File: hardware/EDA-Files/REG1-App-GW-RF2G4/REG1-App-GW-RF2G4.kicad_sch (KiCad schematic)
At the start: 4 parts, among them J1 REG1_App_Connector, U1 E01-ML01DP5, U2 E01-2G4M27S, U3 E07-M1101D-TH

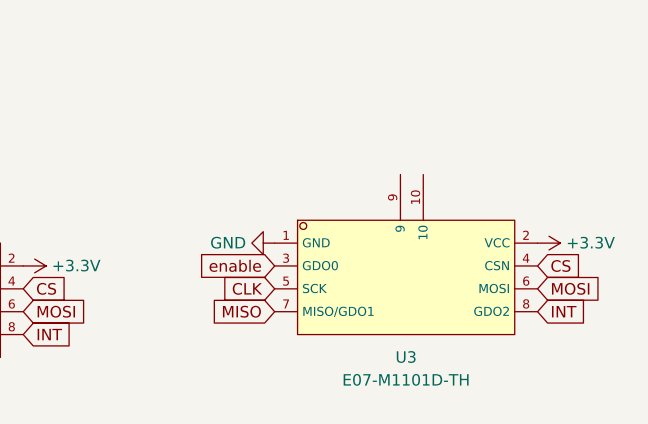
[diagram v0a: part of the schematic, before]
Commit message: wip GW RF
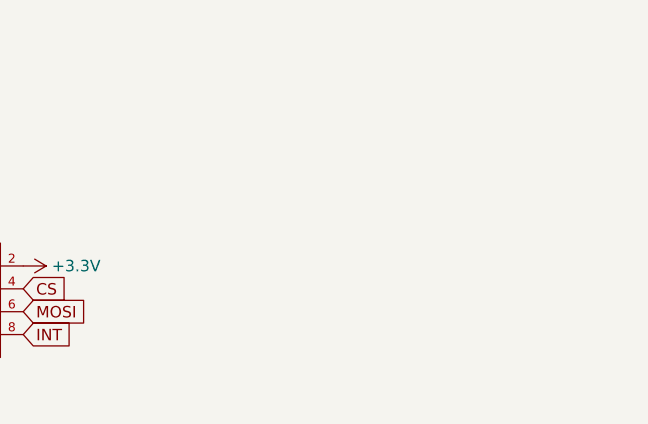
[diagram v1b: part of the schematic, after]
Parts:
- removed U3: E07-M1101D-TH, EasyEDALib:WIRELM-TH_E07-M1101D-TH, symbol EasyEDALib:E07-M1101D-TH
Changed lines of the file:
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@@
     (company "OpenKNX")
     (comment 1 "by Ing-Dom <dom@ing-dom.de>")
+    (comment 2 "OpenKNX Open Hardware under CC BY-NC-SA 4.0")
     (comment 3 "REG1-Application PCB for a 2.4GHz RF module featuring NRF24L01+ chipset")
     (comment 4 "https://OpenKNX.de")
@@
     )
   )
-  (global_label "MOSI" (shape input) (at 237.49 85.09 0) (fields_autoplaced)
-    (effects (font (size 1.27 1.27)) (justify left))
-    (property "Intersheetrefs" "${INTERSHEET_REFS}" (at 244.4172 85.09 0)
-      (effects (font (size 1.27 1.27)) (justify left) hide)
-    )
-  )
-  (global_label "INT" (shape input) (at 237.49 87.63 0) (fields_autoplaced)
-    (effects (font (size 1.27 1.27)) (justify left))
-    (property "Intersheetrefs" "${INTERSHEET_REFS}" (at 242.7239 87.63 0)
-      (effects (font (size 1.27 1.27)) (justify left) hide)
-    )
-  )
   (global_label "INT" (shape input) (at 87.63 45.72 0) (fields_autoplaced)
     (effects (font (size 1.27 1.27)) (justify left))
@@
     )
   )
-  (global_label "enable" (shape input) (at 208.28 82.55 180) (fields_autoplaced)
-    (effects (font (size 1.27 1.27)) (justify right))
-    (property "Intersheetrefs" "${INTERSHEET_REFS}" (at 199.6596 82.55 0)
-      (effects (font (size 1.27 1.27)) (justify right) hide)
-    )
-  )
   (global_label "enable" (shape input) (at 156.21 38.1 180) (fields_autoplaced)
     (effects (font (size 1.27 1.27)) (justify right))
@@
     )
   )
-  (global_label "CS" (shape input) (at 237.49 82.55 0) (fields_autoplaced)
-    (effects (font (size 1.27 1.27)) (justify left))
-    (property "Intersheetrefs" "${INTERSHEET_REFS}" (at 242.3005 82.55 0)
-      (effects (font (size 1.27 1.27)) (justify left) hide)
-    )
-  )
   (global_label "CS" (shape input) (at 87.63 55.88 0) (fields_autoplaced)
     (effects (font (size 1.27 1.27)) (justify left))
@@
     )
   )
-  (global_label "CLK" (shape input) (at 208.28 85.09 180) (fields_autoplaced)
-    (effects (font (size 1.27 1.27)) (justify right))
-    (property "Intersheetrefs" "${INTERSHEET_REFS}" (at 202.3809 85.09 0)
-      (effects (font (size 1.27 1.27)) (justify right) hide)
-    )
-  )
   (global_label "MISO" (shape input) (at 146.05 90.17 180) (fields_autoplaced)
     (effects (font (size 1.27 1.27)) (justify right))
     (property "Intersheetrefs" "${INTERSHEET_REFS}" (at 139.1228 90.17 0)
-      (effects (font (size 1.27 1.27)) (justify right) hide)
-    )
-  )
-  (global_label "MISO" (shape input) (at 208.28 87.63 180) (fields_autoplaced)
-    (effects (font (size 1.27 1.27)) (justify right))
-    (property "Intersheetrefs" "${INTERSHEET_REFS}" (at 201.3528 87.63 0)
       (effects (font (size 1.27 1.27)) (justify right) hide)
     )
@@
     )
   )
-  (symbol (lib_id "power:+3.3V") (at 237.49 80.01 270) (unit 1)
-    (in_bom yes) (on_board yes) (dnp no) (fields_autoplaced)
-    (property "Reference" "#PWR08" (at 233.68 80.01 0)
-      (effects (font (size 1.27 1.27)) hide)
-    )
-    (property "Value" "+3.3V" (at 240.665 80.01 90)
-      (effects (font (size 1.27 1.27)) (justify left))
-    )
-    (property "Footprint" "" (at 237.49 80.01 0)
-      (effects (font (size 1.27 1.27)) hide)
-    )
-    (property "Datasheet" "" (at 237.49 80.01 0)
-      (effects (font (size 1.27 1.27)) hide)
-    )
-    (pin "1")
-    (instances
-      (project "REG1-App-GW-RF2G4"
-        (path "/8b58e694-2557-4422-b559-288aecb40f90"
-          (reference "#PWR08") (unit 1)
-        )
-      )
-    )
-  )
   (symbol (lib_id "power:GND") (at 87.63 58.42 90) (unit 1)
     (in_bom yes) (on_board yes) (dnp no) (fields_autoplaced)
@@
     )
   )
-  (symbol (lib_id "EasyEDALib:E07-M1101D-TH") (at 223.52 83.82 0) (unit 1)
-    (in_bom yes) (on_board yes) (dnp no) (fields_autoplaced)
-    (property "Reference" "U3" (at 222.885 92.71 0)
-      (effects (font (size 1.27 1.27)))
-    )
-    (property "Value" "E07-M1101D-TH" (at 222.885 95.25 0)
-      (effects (font (size 1.27 1.27)))
-    )
-    (property "Footprint" "EasyEDALib:WIRELM-TH_E07-M1101D-TH" (at 223.52 93.98 0)
-      (effects (font (size 1.27 1.27) italic) hide)
-    )
-    (property "Datasheet" "https://item.szlcsc.com/109768.html" (at 221.234 83.693 0)
-      (effects (font (size 1.27 1.27)) (justify left) hide)
-    )
-    (property "LCSC" "C108549" (at 223.52 83.82 0)
+  (symbol (lib_id "power:+3.3V") (at 180.34 82.55 270) (unit 1)
+    (in_bom yes) (on_board yes) (dnp no) (fields_autoplaced)
+    (property "Reference" "#PWR05" (at 176.53 82.55 0)
+      (effects (font (size 1.27 1.27)) hide)
+    )
+    (property "Value" "+3.3V" (at 183.515 82.55 90)
+      (effects (font (size 1.27 1.27)) (justify left))
+    )
+    (property "Footprint" "" (at 180.34 82.55 0)
+      (effects (font (size 1.27 1.27)) hide)
+    )
+    (property "Datasheet" "" (at 180.34 82.55 0)
+      (effects (font (size 1.27 1.27)) hide)
+    )
+    (pin "1")
+    (instances
+      (project "REG1-App-GW-RF2G4"
+        (path "/8b58e694-2557-4422-b559-288aecb40f90"
+          (reference "#PWR05") (unit 1)
+        )
+      )
+    )
+  )
+  (symbol (lib_id "EasyEDAModLib:C2971732_E01-2G4M27S") (at 161.29 43.18 90) (unit 1)
+    (in_bom yes) (on_board yes) (dnp no) (fields_autoplaced)
+    (property "Reference" "U2" (at 167.005 42.6029 90)
+      (effects (font (size 1.27 1.27)) (justify right))
+    )
+    (property "Value" "E01-2G4M27S" (at 167.005 45.0271 90)
+      (effects (font (size 1.27 1.27)) (justify right))
+    )
+    (property "Footprint" "EasyEDAModLib:C2971732_WIRELM-SMD_10P-L23.0-W14.0-P1.27_E01-2G4M27S_Handsolder" (at 170.18 43.18 0)
+      (effects (font (size 1.27 1.27)) hide)
+    )
+    (property "Datasheet" "" (at 161.29 43.18 0)
+      (effects (font (size 1.27 1.27)) hide)
+    )
+    (property "LCSC Part" "C2971732" (at 172.72 43.18 0)
       (effects (font (size 1.27 1.27)) hide)
     )
@@
       (project "REG1-App-GW-RF2G4"
         (path "/8b58e694-2557-4422-b559-288aecb40f90"
-          (reference "U3") (unit 1)
-        )
-      )
-    )
-  )
-  (symbol (lib_id "power:+3.3V") (at 180.34 82.55 270) (unit 1)
-    (in_bom yes) (on_board yes) (dnp no) (fields_autoplaced)
-    (property "Reference" "#PWR05" (at 176.53 82.55 0)
-      (effects (font (size 1.27 1.27)) hide)
-    )
-    (property "Value" "+3.3V" (at 183.515 82.55 90)
-      (effects (font (size 1.27 1.27)) (justify left))
-    )
-    (property "Footprint" "" (at 180.34 82.55 0)
-      (effects (font (size 1.27 1.27)) hide)
-    )
-    (property "Datasheet" "" (at 180.34 82.55 0)
-      (effects (font (size 1.27 1.27)) hide)
-    )
-    (pin "1")
-    (instances
-      (project "REG1-App-GW-RF2G4"
-        (path "/8b58e694-2557-4422-b559-288aecb40f90"
-          (reference "#PWR05") (unit 1)
-        )
-      )
-    )
-  )
-  (symbol (lib_id "EasyEDAModLib:C2971732_E01-2G4M27S") (at 161.29 43.18 90) (unit 1)
-    (in_bom yes) (on_board yes) (dnp no) (fields_autoplaced)
-    (property "Reference" "U2" (at 167.005 42.6029 90)
-      (effects (font (size 1.27 1.27)) (justify right))
-    )
-    (property "Value" "E01-2G4M27S" (at 167.005 45.0271 90)
-      (effects (font (size 1.27 1.27)) (justify right))
-    )
-    (property "Footprint" "EasyEDAModLib:C2971732_WIRELM-SMD_10P-L23.0-W14.0-P1.27_E01-2G4M27S_Handsolder" (at 170.18 43.18 0)
-      (effects (font (size 1.27 1.27)) hide)
-    )
-    (property "Datasheet" "" (at 161.29 43.18 0)
-      (effects (font (size 1.27 1.27)) hide)
-    )
-    (property "LCSC Part" "C2971732" (at 172.72 43.18 0)
-      (effects (font (size 1.27 1.27)) hide)
-    )
-    (pin "1")
-    (pin "10")
-    (pin "2")
-    (pin "3")
-    (pin "4")
-    (pin "5")
-    (pin "6")
-    (pin "7")
-    (pin "8")
-    (pin "9")
-    (instances
-      (project "REG1-App-GW-RF2G4"
-        (path "/8b58e694-2557-4422-b559-288aecb40f90"
           (reference "U2") (unit 1)
         )
@@
         )
       )
-    )
-  )
-  (symbol (lib_id "power:GND") (at 208.28 80.01 270) (unit 1)
-    (in_bom yes) (on_board yes) (dnp no) (fields_autoplaced)
-    (property "Reference" "#PWR07" (at 201.93 80.01 0)
-      (effects (font (size 1.27 1.27)) hide)
-    )
-    (property "Value" "GND" (at 205.1051 80.01 90)
-      (effects (font (size 1.27 1.27)) (justify right))
-    )
-    (property "Footprint" "" (at 208.28 80.01 0)
-      (effects (font (size 1.27 1.27)) hide)
-    )
-    (property "Datasheet" "" (at 208.28 80.01 0)
-      (effects (font (size 1.27 1.27)) hide)
-    )
-    (pin "1")
-    (instances
-      (project "REG1-App-GW-RF2G4"
-        (path "/8b58e694-2557-4422-b559-288aecb40f90"
-          (reference "#PWR07") (unit 1)
-        )
-      )

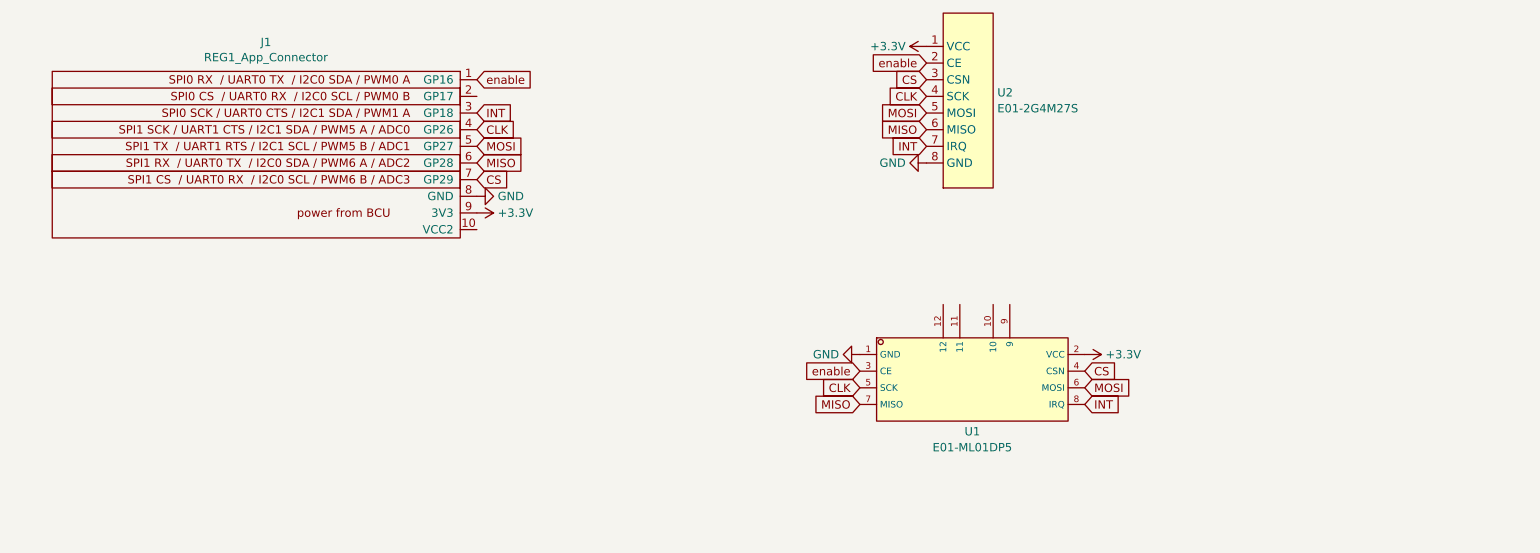
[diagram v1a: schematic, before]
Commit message: App-GW-RF2G4 V00.01
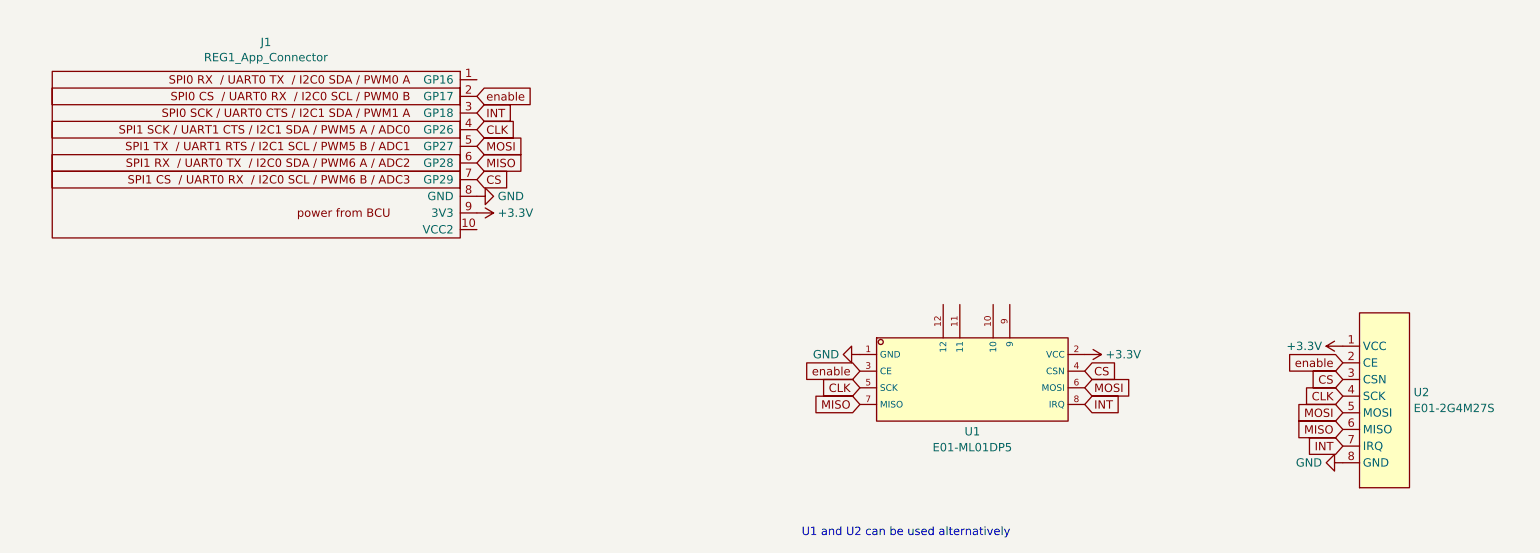
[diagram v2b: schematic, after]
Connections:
- net enable: now also J1.2 (GP17); no longer J1.1 (GP16)
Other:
- note added: "U1 and U2 can be used alternatively"
- moved on the sheet: U2
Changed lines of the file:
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@@
   (title_block
     (title "REG1-App-GW-RF2G4")
-    (date "2024-07-25")
+    (date "2024-07-29")
     (rev "V00.01")
     (company "OpenKNX")
@@
     (comment 4 "https://OpenKNX.de")
   )
-  (global_label "MOSI" (shape input) (at 156.21 45.72 180) (fields_autoplaced)
-    (effects (font (size 1.27 1.27)) (justify right))
-    (property "Intersheetrefs" "${INTERSHEET_REFS}" (at 149.2828 45.72 0)
+  (text "U1 and U2 can be used alternatively" (at 137.16 110.49 0)
+    (effects (font (size 1.27 1.27)) (justify left bottom))
+  )
+  (global_label "MOSI" (shape input) (at 219.71 91.44 180) (fields_autoplaced)
+    (effects (font (size 1.27 1.27)) (justify right))
+    (property "Intersheetrefs" "${INTERSHEET_REFS}" (at 212.7828 91.44 0)
       (effects (font (size 1.27 1.27)) (justify right) hide)
     )
@@
     )
   )
-  (global_label "INT" (shape input) (at 156.21 50.8 180) (fields_autoplaced)
-    (effects (font (size 1.27 1.27)) (justify right))
-    (property "Intersheetrefs" "${INTERSHEET_REFS}" (at 150.9761 50.8 0)
+  (global_label "INT" (shape input) (at 219.71 96.52 180) (fields_autoplaced)
+    (effects (font (size 1.27 1.27)) (justify right))
+    (property "Intersheetrefs" "${INTERSHEET_REFS}" (at 214.4761 96.52 0)
       (effects (font (size 1.27 1.27)) (justify right) hide)
     )
@@
     )
   )
-  (global_label "enable" (shape input) (at 87.63 40.64 0) (fields_autoplaced)
-    (effects (font (size 1.27 1.27)) (justify left))
-    (property "Intersheetrefs" "${INTERSHEET_REFS}" (at 96.2504 40.64 0)
+  (global_label "enable" (shape input) (at 87.63 43.18 0) (fields_autoplaced)
+    (effects (font (size 1.27 1.27)) (justify left))
+    (property "Intersheetrefs" "${INTERSHEET_REFS}" (at 96.2504 43.18 0)
       (effects (font (size 1.27 1.27)) (justify left) hide)
     )
@@
     )
   )
-  (global_label "CS" (shape input) (at 156.21 40.64 180) (fields_autoplaced)
-    (effects (font (size 1.27 1.27)) (justify right))
-    (property "Intersheetrefs" "${INTERSHEET_REFS}" (at 151.3995 40.64 0)
-      (effects (font (size 1.27 1.27)) (justify right) hide)
-    )
-  )
-  (global_label "MISO" (shape input) (at 156.21 48.26 180) (fields_autoplaced)
-    (effects (font (size 1.27 1.27)) (justify right))
-    (property "Intersheetrefs" "${INTERSHEET_REFS}" (at 149.2828 48.26 0)
+  (global_label "CS" (shape input) (at 219.71 86.36 180) (fields_autoplaced)
+    (effects (font (size 1.27 1.27)) (justify right))
+    (property "Intersheetrefs" "${INTERSHEET_REFS}" (at 214.8995 86.36 0)
+      (effects (font (size 1.27 1.27)) (justify right) hide)
+    )
+  )
+  (global_label "MISO" (shape input) (at 219.71 93.98 180) (fields_autoplaced)
+    (effects (font (size 1.27 1.27)) (justify right))
+    (property "Intersheetrefs" "${INTERSHEET_REFS}" (at 212.7828 93.98 0)
       (effects (font (size 1.27 1.27)) (justify right) hide)
     )
@@
     )
   )
-  (global_label "CLK" (shape input) (at 156.21 43.18 180) (fields_autoplaced)
-    (effects (font (size 1.27 1.27)) (justify right))
-    (property "Intersheetrefs" "${INTERSHEET_REFS}" (at 150.3109 43.18 0)
+  (global_label "CLK" (shape input) (at 219.71 88.9 180) (fields_autoplaced)
+    (effects (font (size 1.27 1.27)) (justify right))
+    (property "Intersheetrefs" "${INTERSHEET_REFS}" (at 213.8109 88.9 0)
       (effects (font (size 1.27 1.27)) (justify right) hide)
     )
@@
     )
   )
-  (global_label "enable" (shape input) (at 156.21 38.1 180) (fields_autoplaced)
-    (effects (font (size 1.27 1.27)) (justify right))
-    (property "Intersheetrefs" "${INTERSHEET_REFS}" (at 147.5896 38.1 0)
+  (global_label "enable" (shape input) (at 219.71 83.82 180) (fields_autoplaced)
+    (effects (font (size 1.27 1.27)) (justify right))
+    (property "Intersheetrefs" "${INTERSHEET_REFS}" (at 211.0896 83.82 0)
       (effects (font (size 1.27 1.27)) (justify right) hide)
     )
@@
     )
   )
-  (symbol (lib_id "EasyEDAModLib:C2971732_E01-2G4M27S") (at 161.29 43.18 90) (unit 1)
-    (in_bom yes) (on_board yes) (dnp no) (fields_autoplaced)
-    (property "Reference" "U2" (at 167.005 42.6029 90)
-      (effects (font (size 1.27 1.27)) (justify right))
-    )
-    (property "Value" "E01-2G4M27S" (at 167.005 45.0271 90)
-      (effects (font (size 1.27 1.27)) (justify right))
-    )
-    (property "Footprint" "EasyEDAModLib:C2971732_WIRELM-SMD_10P-L23.0-W14.0-P1.27_E01-2G4M27S_Handsolder" (at 170.18 43.18 0)
-      (effects (font (size 1.27 1.27)) hide)
-    )
-    (property "Datasheet" "" (at 161.29 43.18 0)
-      (effects (font (size 1.27 1.27)) hide)
-    )
-    (property "LCSC Part" "C2971732" (at 172.72 43.18 0)
+  (symbol (lib_id "EasyEDAModLib:C2971732_E01-2G4M27S") (at 224.79 88.9 90) (unit 1)
+    (in_bom yes) (on_board yes) (dnp no) (fields_autoplaced)
+    (property "Reference" "U2" (at 230.505 88.3229 90)
+      (effects (font (size 1.27 1.27)) (justify right))
+    )
+    (property "Value" "E01-2G4M27S" (at 230.505 90.7471 90)
+      (effects (font (size 1.27 1.27)) (justify right))
+    )
+    (property "Footprint" "EasyEDAModLib:C2971732_WIRELM-SMD_10P-L23.0-W14.0-P1.27_E01-2G4M27S_Handsolder" (at 233.68 88.9 0)
+      (effects (font (size 1.27 1.27)) hide)
+    )
+    (property "Datasheet" "" (at 224.79 88.9 0)
+      (effects (font (size 1.27 1.27)) hide)
+    )
+    (property "LCSC Part" "C2971732" (at 236.22 88.9 0)
       (effects (font (size 1.27 1.27)) hide)
     )
@@
     )
   )
-  (symbol (lib_id "power:GND") (at 156.21 53.34 270) (unit 1)
-    (in_bom yes) (on_board yes) (dnp no) (fields_autoplaced)
-    (property "Reference" "#PWR02" (at 149.86 53.34 0)
-      (effects (font (size 1.27 1.27)) hide)
-    )
-    (property "Value" "GND" (at 153.0351 53.34 90)
-      (effects (font (size 1.27 1.27)) (justify right))
-    )
-    (property "Footprint" "" (at 156.21 53.34 0)
-      (effects (font (size 1.27 1.27)) hide)
-    )
-    (property "Datasheet" "" (at 156.21 53.34 0)
+  (symbol (lib_id "power:GND") (at 219.71 99.06 270) (unit 1)
+    (in_bom yes) (on_board yes) (dnp no) (fields_autoplaced)
+    (property "Reference" "#PWR02" (at 213.36 99.06 0)
+      (effects (font (size 1.27 1.27)) hide)
+    )
+    (property "Value" "GND" (at 216.5351 99.06 90)
+      (effects (font (size 1.27 1.27)) (justify right))
+    )
+    (property "Footprint" "" (at 219.71 99.06 0)
+      (effects (font (size 1.27 1.27)) hide)
+    )
+    (property "Datasheet" "" (at 219.71 99.06 0)
       (effects (font (size 1.27 1.27)) hide)
     )
@@
     )
   )
-  (symbol (lib_id "power:+3.3V") (at 156.21 35.56 90) (unit 1)
-    (in_bom yes) (on_board yes) (dnp no) (fields_autoplaced)
-    (property "Reference" "#PWR06" (at 160.02 35.56 0)
-      (effects (font (size 1.27 1.27)) hide)
-    )
-    (property "Value" "+3.3V" (at 153.035 35.56 90)
+  (symbol (lib_id "power:+3.3V") (at 219.71 81.28 90) (unit 1)
+    (in_bom yes) (on_board yes) (dnp no) (fields_autoplaced)
+    (property "Reference" "#PWR06" (at 223.52 81.28 0)
+      (effects (font (size 1.27 1.27)) hide)
+    )
+    (property "Value" "+3.3V" (at 216.535 81.28 90)
       (effects (font (size 1.27 1.27)) (justify left))
     )
-    (property "Footprint" "" (at 156.21 35.56 0)
-      (effects (font (size 1.27 1.27)) hide)
-    )
-    (property "Datasheet" "" (at 156.21 35.56 0)
-      (effects (font (size 1.27 1.27)) hide)
-    )
+    (property "Footprint" "" (at 219.71 81.28 0)
+      (effects (font (size 1.27 1.27)) hide)
+    )
+    (property "Datasheet" "" (at 219.71 81.28 0)
+      (effects (font (size 1.27 1.27)) hide)
+    )
